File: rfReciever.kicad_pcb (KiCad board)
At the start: 4 copper layers, 33.8 x 20.5 mm, 38 parts, among them J1 MOLEX 1054440001, SW1 RF_RESET, SW2 RF_SLEEP, U1 CP2102N-A02-GQFN24, U2 USBLC6-2SC6, X1 DigiXBeeRX900Micro

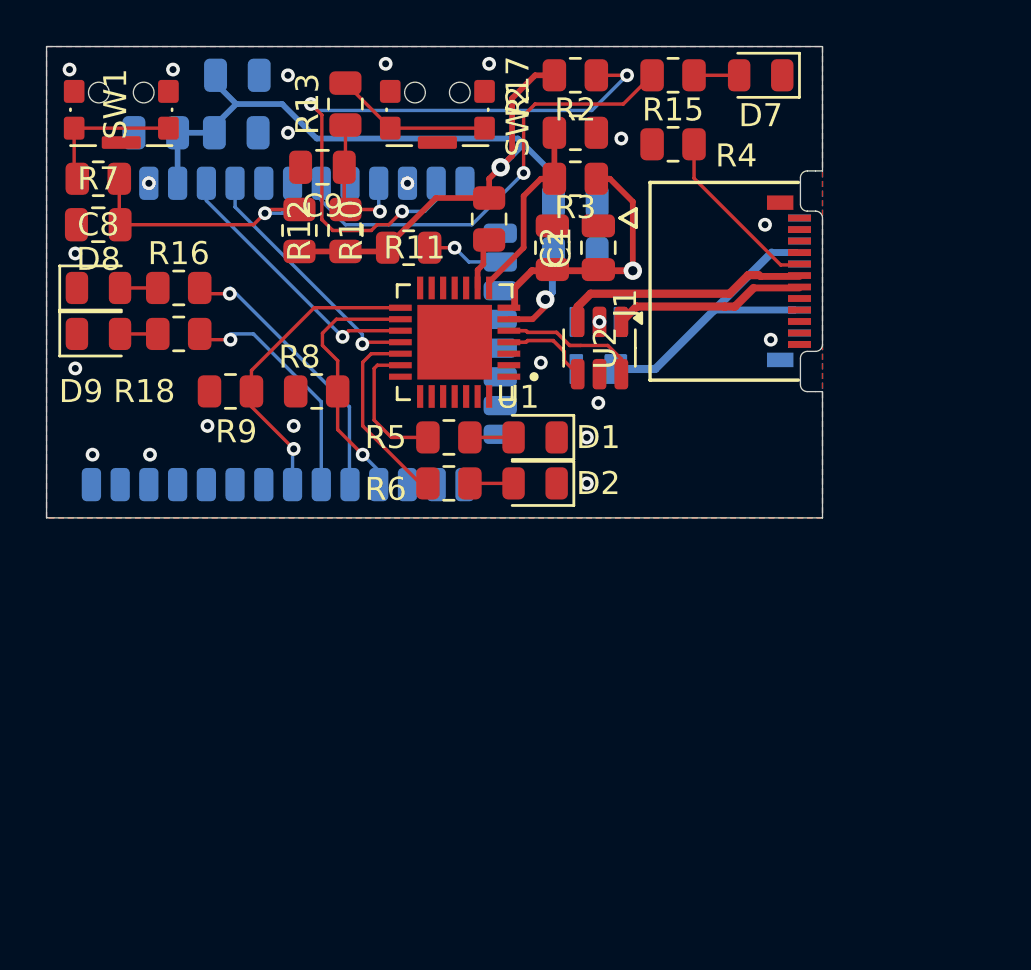
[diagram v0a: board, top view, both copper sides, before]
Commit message: fixed traces and errors
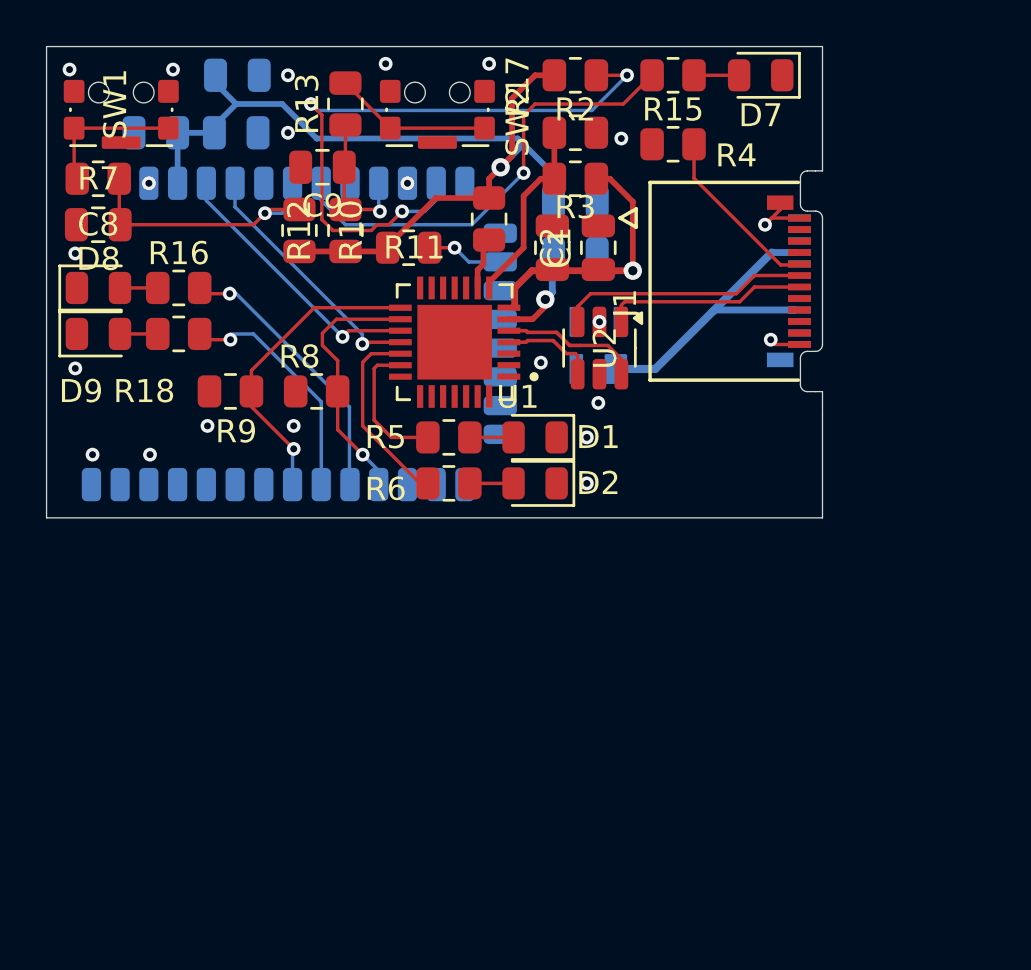
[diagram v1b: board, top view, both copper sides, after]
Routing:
- net GND: track 0.00 -> 4.19 mm
- removed copper zone on B.Cu, net +5V
- removed copper zone on F.Cu, net +5V
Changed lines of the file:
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@@
 		(layer "Edge.Cuts")
+	)
+	(segment
+		(start 126.29125 67.95875)
+		(end 126 68.25)
+		(width 0.15)
+		(layer "F.Cu")
+		(net 1)
+	)
+	(segment
+		(start 126.45875 73.45875)
+		(end 126.25 73.25)
+		(width 0.15)
+		(layer "F.Cu")
+		(net 1)
+	)
+	(segment
+		(start 127.5 73.45875)
+		(end 126.45875 73.45875)
+		(width 0.15)
+		(layer "F.Cu")
+		(net 1)
+	)
+	(segment
+		(start 127.5 67.95875)
+		(end 126.29125 67.95875)
+		(width 0.15)
+		(layer "F.Cu")
+		(net 1)
+	)
+	(segment
+		(start 126.66 67.59)
+		(end 126 68.25)
+		(width 0.15)
+		(layer "F.Cu")
+		(net 1)
+	)
+	(segment
+		(start 126.66 67.28875)
+		(end 126.66 67.59)
+		(width 0.15)
+		(layer "F.Cu")
+		(net 1)
 	)
 	(via
@@
 	)
 	(segment
-		(start 124.25 71.81)
-		(end 124.69 71.81)
-		(width 0.36)
+		(start 127.5 70.95875)
+		(end 125.54125 70.95875)
+		(width 0.15)
 		(layer "F.Cu")
 		(net 43)
 	)
 	(segment
-		(start 124.69 71.81)
-		(end 125.5 71)
-		(width 0.36)
+		(start 124.9 71.6)
+		(end 119.9 71.6)
+		(width 0.15)
 		(layer "F.Cu")
 		(net 43)
 	)
 	(segment
-		(start 120.415 71.81)
-		(end 124.25 71.81)
-		(width 0.36)
+		(start 125.54125 70.95875)
+		(end 124.9 71.6)
+		(width 0.15)
 		(layer "F.Cu")
 		(net 43)
 	)
 	(segment
-		(start 127.5 71)
-		(end 125.5 71)
-		(width 0.3)
+		(start 119.9 71.6)
+		(end 119.75 71.75)
+		(width 0.15)
 		(layer "F.Cu")
 		(net 43)
 	)
 	(segment
-		(start 119.75 72.475)
-		(end 120.415 71.81)
-		(width 0.36)
+		(start 119.75 71.75)
+		(end 119.75 72.475)
+		(width 0.15)
 		(layer "F.Cu")
 		(net 43)
 	)
 	(segment
-		(start 124.45804 71.25)
-		(end 125.26804 70.44)
-		(width 0.36)
+		(start 125.54125 70.45875)
+		(end 124.75 71.25)
+		(width 0.15)
 		(layer "F.Cu")
 		(net 44)
 	)
 	(segment
-		(start 125.79196 70.5)
-		(end 125.73196 70.44)
-		(width 0.3)
+		(start 124.75 71.25)
+		(end 118.412501 71.25)
+		(width 0.15)
 		(layer "F.Cu")
 		(net 44)
 	)
 	(segment
-		(start 127.5 70.5)
-		(end 125.79196 70.5)
-		(width 0.3)
+		(start 118.412501 71.25)
+		(end 117.85 71.812501)
+		(width 0.15)
 		(layer "F.Cu")
 		(net 44)
 	)
 	(segment
-		(start 118.412501 71.25)
-		(end 124.45804 71.25)
-		(width 0.36)
+		(start 117.85 71.812501)
+		(end 117.85 72.475)
+		(width 0.15)
 		(layer "F.Cu")
 		(net 44)
 	)
 	(segment
-		(start 117.85 72.475)
-		(end 117.85 71.812501)
-		(width 0.36)
-		(layer "F.Cu")
-		(net 44)
-	)
-	(segment
-		(start 125.26804 70.44)
-		(end 125.73196 70.44)
-		(width 0.36)
-		(layer "F.Cu")
-		(net 44)
-	)
-	(segment
-		(start 117.85 71.812501)
-		(end 118.412501 71.25)
-		(width 0.36)
+		(start 127.5 70.45875)
+		(end 125.54125 70.45875)
+		(width 0.15)
 		(layer "F.Cu")
 		(net 44)
@@
 	)
 	(segment
-		(start 117.270957 74.170957)
-		(end 117.85 74.75)
-		(width 0.15)
-		(layer "F.Cu")
-		(net 46)
-	)
-	(segment
-		(start 117.270957 73.773749)
-		(end 117.270957 74.170957)
+		(start 117.85 73.95375)
+		(end 117.75 73.85375)
 		(width 0.15)
 		(layer "F.Cu")
@@
 	)
 	(segment
+		(start 117.75 73.85375)
+		(end 117.356264 73.85375)
+		(width 0.15)
+		(layer "F.Cu")
+		(net 46)
+	)
+	(segment
 		(start 115.673751 73.28875)
 		(end 116.785958 73.28875)
@@
 	)
 	(segment
+		(start 117.85 74.75)
+		(end 117.85 73.95375)
+		(width 0.15)
+		(layer "F.Cu")
+		(net 46)
+	)
+	(segment
 		(start 115.602501 73.36)
 		(end 115.673751 73.28875)
@@
 	)
 	(segment
+		(start 117.276263 73.773749)
+		(end 117.270957 73.773749)
+		(width 0.15)
+		(layer "F.Cu")
+		(net 46)
+	)
+	(segment
+		(start 117.356264 73.85375)
+		(end 117.276263 73.773749)
+		(width 0.15)
+		(layer "F.Cu")
+		(net 46)
+	)
+	(segment
 		(start 119.162499 73.5)
 		(end 119.75 74.087501)
@@
 	)
 	(zone
-		(net 36)
-		(net_name "+5V")
-		(layers "F&B.Cu")
-		(hatch edge 0.5)
-		(priority 1)
-		(connect_pads
-			(clearance 0.5)
-		)
-		(min_thickness 0.25)
-		(filled_areas_thickness no)
-		(fill yes
-			(thermal_gap 0.5)
-			(thermal_bridge_width 0.5)
-		)
-		(polygon
-			(pts
-				(xy 94.75 60.5) (xy 128.5 60.5) (xy 128.5 81) (xy 94.75 81)
-			)
-		)
-	)
-	(zone

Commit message: reworked schematic v1 matthew review
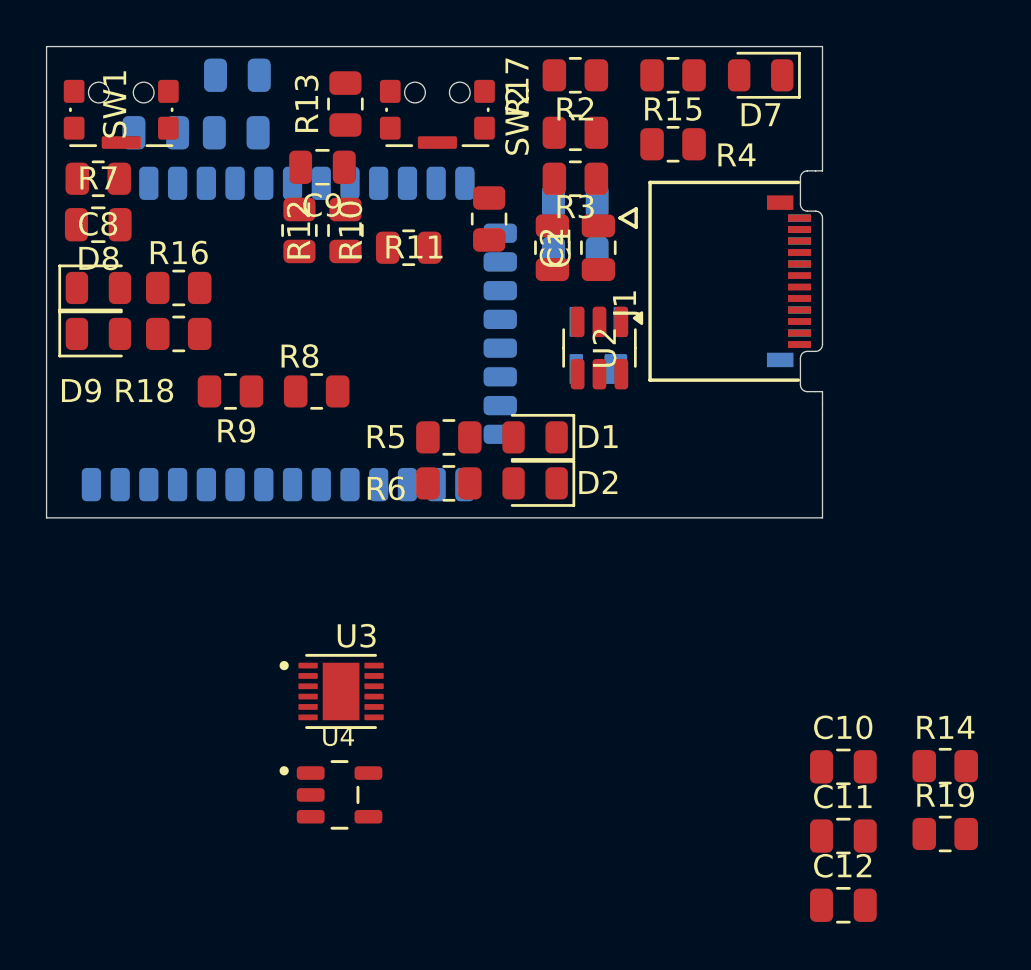
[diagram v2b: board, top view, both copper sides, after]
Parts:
- removed U1: CP2102N-A02-GQFN24, rfReciever-Footprints:QFN50P500X500X80-29N
- added C10: 1uF, Capacitor_SMD:C_0805_2012Metric, F.Cu at (129.4, 91.8)
- added C11: 4.7uF, Capacitor_SMD:C_0805_2012Metric, F.Cu at (129.4, 94.8)
- added C12: 0.1uF, Capacitor_SMD:C_0805_2012Metric, F.Cu at (129.4, 97.8)
- added R14: 27, Resistor_SMD:R_0805_2012Metric, F.Cu at (133.8, 91.8)
- added R19: 27, Resistor_SMD:R_0805_2012Metric, F.Cu at (133.8, 94.8)
- added U3: FT234XD-R, rfReciever-Footprints:SON45P300X300X80-13N, F.Cu at (107.6, 88.5)
- added U4: TPS76333DBVT, rfReciever-Footprints:SOT95P280X145-5N, F.Cu at (107.5, 93.0)
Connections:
- J1 pad A4: /MLX(VBUS) -> +5V
- J1 pad A9: /MLX(VBUS) -> +5V
- J1 pad B4: /MLX(VBUS) -> +5V
- J1 pad B9: /MLX(VBUS) -> +5V
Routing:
- net +3.3V: track 48.4 -> 0.00 mm, vias 2 -> 0
- net /RF_BOOTMODE: track 27.5 -> 0.00 mm, vias 3 -> 0
- net /RF_PWM: track 19.7 -> 0.00 mm, vias 1 -> 0
- net /MLX(VBUS): track 13.5 -> 0.00 mm
- net /UART_CTS: track 13.4 -> 0.00 mm, vias 1 -> 0
- net /RF_RESET: track 12.6 -> 0.00 mm, vias 1 -> 0
- net /RF_DSLEEP: track 12.1 -> 0.00 mm, vias 1 -> 0
- net /RF_RXD: track 11.8 -> 0.00 mm, vias 1 -> 0
- net +5V: track 11.3 -> 0.00 mm, vias 1 -> 0
- net /UART_RTS: track 11.2 -> 0.00 mm, vias 1 -> 0
- net /RF_TXD: track 11.0 -> 0.00 mm, vias 1 -> 0
- net /MLX(D+): track 10.9 -> 0.00 mm
- net /RF_ASSOCIATE: track 10.2 -> 0.00 mm, vias 1 -> 0
- net /MLX(D-): track 8.80 -> 0.00 mm
- net Net-(U1-~{RXT}/GPIO.3): track 8.43 -> 0.00 mm
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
